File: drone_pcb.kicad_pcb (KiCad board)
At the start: 4 copper layers, 52.5 x 52.5 mm, 35 parts, among them J1 HappyModel EP1, J10 M4_NEG, J2 BATT, J3 M1_NEG, J4 M1_POS, J5 M2_POS, J6 M2_NEG, J7 M3_POS, J8 M3_NEG, J9 M4_POS, Q1 AO3400A, Q2 AO3400A, Q3 AO3400A, Q4 AO3400A, U1 OC09600, U2 AP2112K-3.3

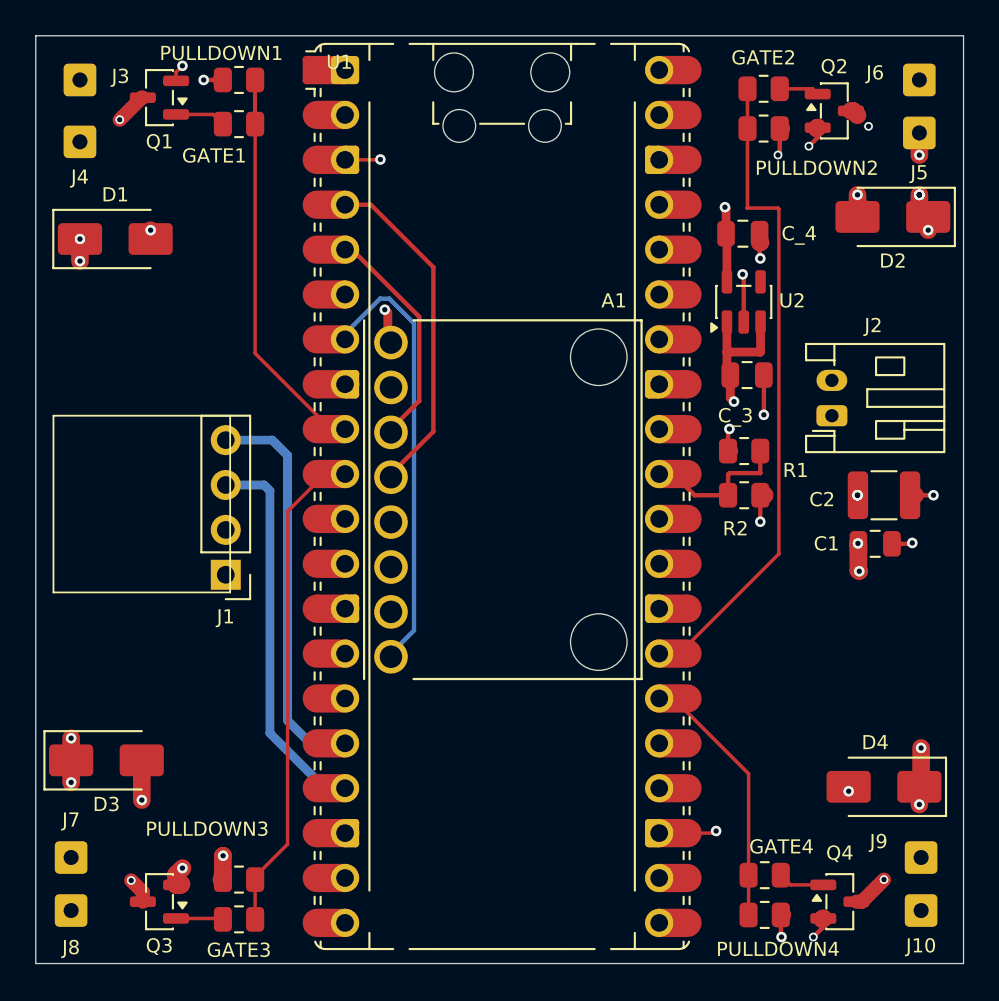
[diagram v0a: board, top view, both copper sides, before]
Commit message: final draft i think
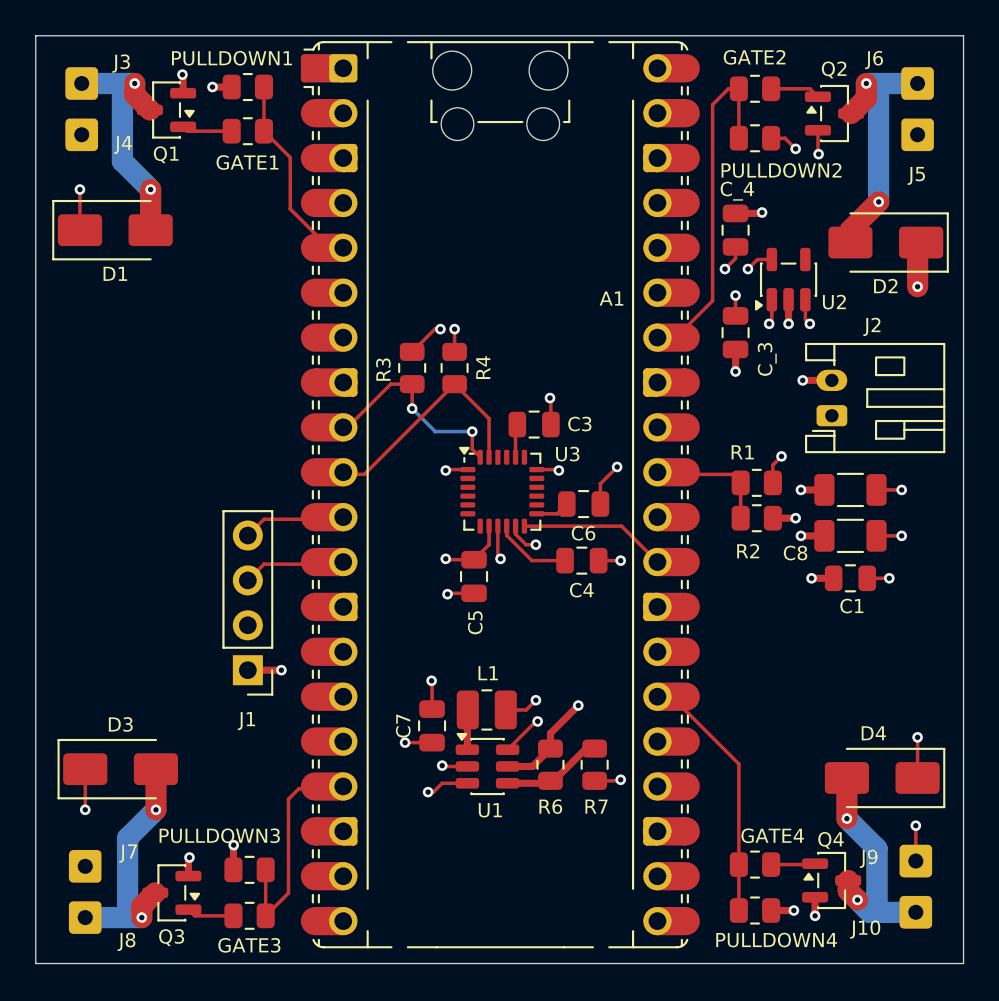
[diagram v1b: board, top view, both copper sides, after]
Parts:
- added C3: 2.2nF, Capacitor_SMD:C_0805_2012Metric, F.Cu at (90.2, 99.0)
- added C4: 0.1uF, Capacitor_SMD:C_0805_2012Metric, F.Cu at (92.9, 106.7)
- added C5: 0.1uF, Capacitor_SMD:C_0805_2012Metric, F.Cu at (86.8, 107.6)
- added C6: 0.1uF, Capacitor_SMD:C_0805_2012Metric, F.Cu at (93.0, 103.5)
- added C7: 22uF, Capacitor_SMD:C_0805_2012Metric, F.Cu at (84.4, 116.0)
- added C8: 100µF, Capacitor_SMD:C_1206_3216Metric, F.Cu at (108.1, 105.3)
- added L1: 2.2uH, Inductor_SMD:L_1008_2520Metric, F.Cu at (87.5, 115.2)
- added R3: 4.7kΩ, Resistor_SMD:R_0805_2012Metric, F.Cu at (83.3, 95.8)
- added R4: 4.7kΩ, Resistor_SMD:R_0805_2012Metric, F.Cu at (85.7, 95.8)
- added R6: 910kΩ, Resistor_SMD:R_0805_2012Metric, F.Cu at (91.1, 118.2)
- added R7: 100kΩ, Resistor_SMD:R_0805_2012Metric, F.Cu at (93.6, 118.2)
- added U3: MPU-6050, Sensor_Motion:InvenSense_QFN-24_4x4mm_P0.5mm, F.Cu at (88.4, 102.8)
- C2: value 220µF -> 100µF; footprint Capacitor_SMD:C_1210_3225Metric -> Capacitor_SMD:C_1206_3216Metric
- U1: value OC09600 -> TLV61070ADBV; footprint OC09600:MODULE_OC09600 -> Package_TO_SOT_SMD:SOT-23-6
- moved U1 15.1 mm to (87.6, 118.3)
- moved J1 5.54 mm to (74.0, 112.9)
- moved U2 2.83 mm to (104.6, 90.8)
- moved C_3 2.49 mm to (101.6, 93.8), turned to -90 degrees
- moved C1 2.40 mm to (108.1, 107.7), turned to 180 degrees
- moved R1 1.94 mm to (102.8, 102.3), turned to 180 degrees
- moved C2 1.92 mm to (108.1, 102.7), turned to 180 degrees
- moved D2 1.50 mm to (110.1, 88.7)
- moved R2 1.48 mm to (102.8, 104.3)
- moved Q4 1.29 mm to (107.0, 124.8)
- moved D3 0.94 mm to (66.8, 118.5)
- moved J7 0.94 mm to (64.8, 124.0)
- moved J8 0.89 mm to (64.8, 126.9)
- moved Q3 0.86 mm to (69.7, 125.5)
- moved GATE4 0.81 mm to (102.7, 123.9)
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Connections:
- A1 pad 10: /M3_PWM -> /IMU_SCL
- A1 pad 11: unconnected-(A1-GPIO8-Pad11) -> /RC_RX
- A1 pad 12: unconnected-(A1-GPIO9-Pad12) -> /RC_TX
- A1 pad 16: /RC_RX -> unconnected-(A1-GPIO12-Pad16)_1
- A1 pad 17: /RC_TX -> /M3_PWM
- A1 pad 27: /M2_PWM -> unconnected-(A1-GPIO21-Pad27)
- A1 pad 29: unconnected-(A1-GPIO22-Pad29)_1 -> /IMU_INT
- A1 pad 34: unconnected-(A1-GPIO28_ADC2-Pad34) -> /M2_PWM
- A1 pad 4: /IMU_SDA -> unconnected-(A1-GPIO2-Pad4)_1
- A1 pad 5: /IMU_SCL -> /M1_PWM
- A1 pad 7: /IMU_INT -> unconnected-(A1-GPIO5-Pad7)
- A1 pad 9: /M1_PWM -> /IMU_SDA
- C_3 pad 1: /PWR -> Net-(U1-V_{OUT})
- C_4 pad 1: Net-(J1-VDD) -> /3.3V
- U2 pad 1: /PWR -> Net-(U1-V_{OUT})
- U2 pad 3: /PWR -> Net-(U1-V_{OUT})
- U2 pad 5: Net-(J1-VDD) -> /3.3V
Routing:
- net /PWR: track 132.3 -> 24.6 mm, vias 17 -> 12
- net Net-(J1-VDD): track 48.8 -> 0.00 mm, vias 2 -> 0
- net /M2_PWM: track 37.2 -> 18.9 mm
- net /IMU_INT: track 25.1 -> 8.54 mm
- net /RC_RX: track 22.6 -> 6.52 mm
- net /RC_TX: track 21.9 -> 5.90 mm
- net /M3_PWM: track 28.0 -> 13.2 mm
- net /M1_PWM: track 24.8 -> 10.8 mm
- net Net-(U1-V_{OUT}): track 0.00 -> 11.6 mm, vias 0 -> 5
- net GND: track 27.6 -> 36.4 mm, vias 16 -> 26
- net Net-(U3-VLOGIC): track 0.00 -> 7.29 mm, vias 0 -> 3
- net /3.3V: track 0.00 -> 7.09 mm, vias 0 -> 4
- net /IMU_SDA: track 19.4 -> 12.6 mm, vias 0 -> 2
- net Net-(U1-V_{FB}): track 0.00 -> 5.74 mm
- net Net-(U3-REGOUT): track 0.00 -> 4.41 mm
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- added copper zone on In2.Cu, net /3.3V
- added copper zone on In2.Cu, net Net-(U1-V_{OUT})
- added copper zone on In2.Cu, net Net-(U3-VLOGIC)
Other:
- board text added: "J9"
- board text added: "awesome drone project"
